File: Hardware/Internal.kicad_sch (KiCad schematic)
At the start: 128 parts, among them J1 SWD, J10 24V_OUT, J11 24V_OUT, J12 24V_OUT, J13 24V_OUT, J14 24V_OUT, J15 CAN, J16 CAN, J17 CAN, J18 CAN, J19 CAN, J2 CAN, J20 CAN, J21 DR16, J22 2.54, J23 2.54, J24 2.54, J3 USB_C_Receptacle_USB2.0, J4 JLINK_SWD, J5 CAN, J6 24V_IN, J7 24V_OUT, J8 24V_OUT, J9 24V_OUT, Q1 S8050, Q2 AO3400A, Q3 AO3400A, SW1 BTN1, SW2 RST, U1 STM32G431CBUx, U2 SIT1042T/3, U3 STM32F103CBT6, U4 RS3236, U5 RY8411, Y1 8MHz, Y3 8MHz

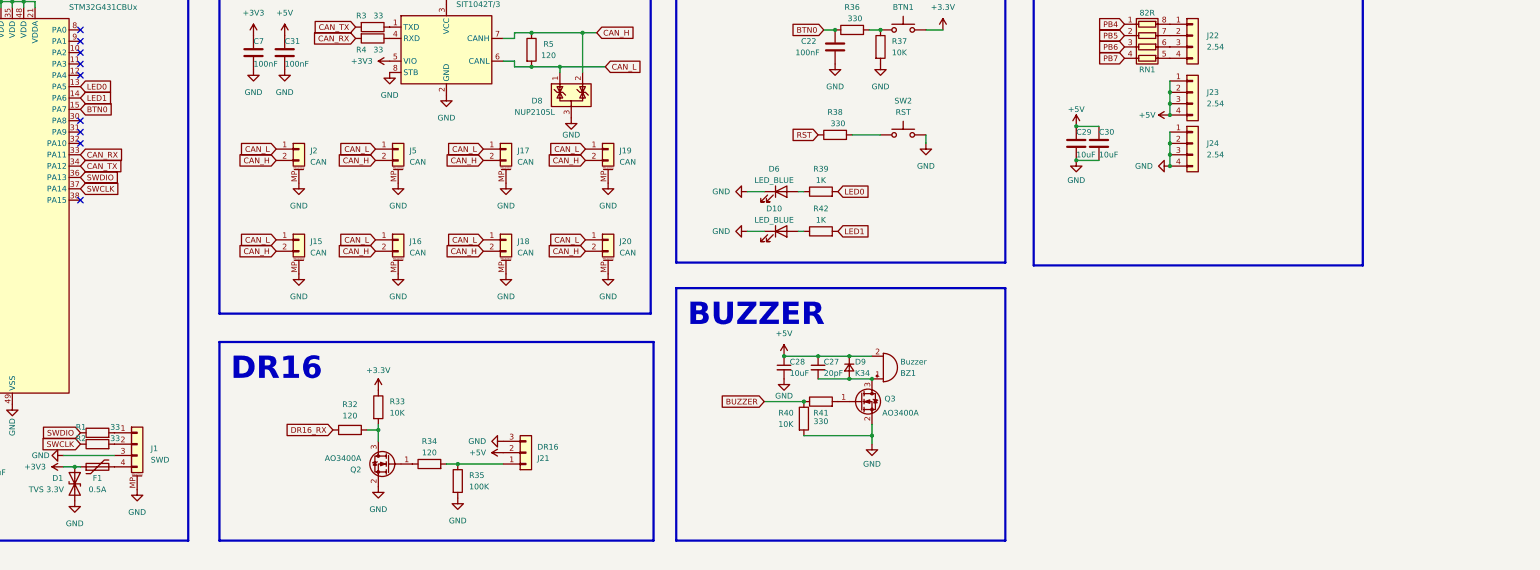
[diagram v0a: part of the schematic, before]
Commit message: update PCB
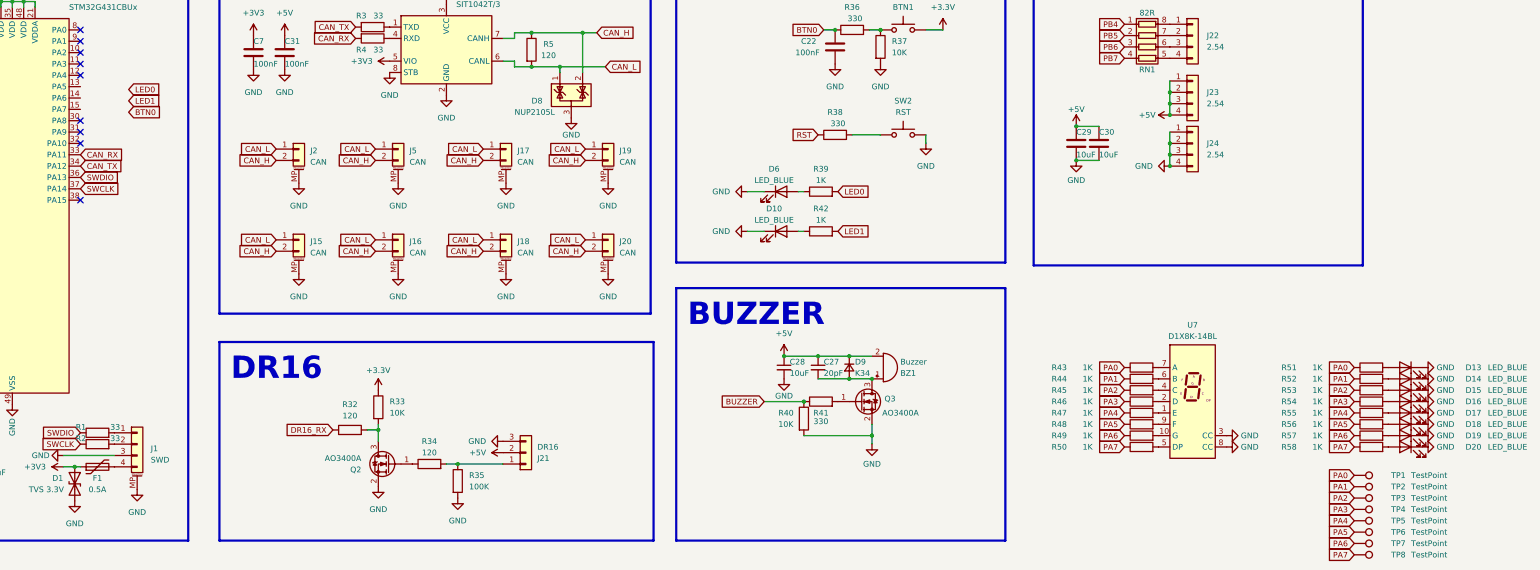
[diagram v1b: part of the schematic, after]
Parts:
- added D13, D14, D15, D16, D17, D18, D19, D20: LED_BLUE, LED_SMD:LED_0603_1608Metric, symbol Device:LED
- added R43, R44, R45, R46, R47, R48, R49, R50, R51, R52, R53, R54, R55, R56, R57, R58: 1K, Resistor_SMD:R_0603_1608Metric, symbol Device:R
- added TP1, TP2, TP3, TP4, TP5, TP6, TP7, TP8: TestPoint, TestPoint:TestPoint_THTPad_2.0x2.0mm_Drill1.0mm, symbol Connector:TestPoint
- added U7: D1X8K-14BL, Display_7Segment:D1X8K, symbol Display_Character:D1X8K-14BL
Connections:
- net BTN0: no longer U1.15 (PA7)
- net GND: now also D13.1 (K), D14.1 (K), D15.1 (K), D16.1 (K), D17.1 (K), D18.1 (K), D19.1 (K), D20.1 (K), U7.3 (CC), U7.8 (CC)
- net LED0: no longer U1.13 (PA5)
- net LED1: no longer U1.14 (PA6)
- new net: D20.2 (A), R58.2
- new net: R48.2, U7.9 (F)
- new net: D19.2 (A), R57.2
- new net: R46.2, U7.2 (D)
- new net: R49.2, U7.10 (G)
- new net: D15.2 (A), R53.2
- new net: R50.2, U7.5 (DP)
- new net: D17.2 (A), R55.2
- new net: D14.2 (A), R52.2
- new net: D13.2 (A), R51.2
- new net: R43.2, U7.7 (A)
- new net: D16.2 (A), R54.2
- new net: R47.2, U7.1 (E)
- new net: R45.2, U7.4 (C)
- new net: R44.2, U7.6 (B)
- new net: D18.2 (A), R56.2
- new net PA0: R43.1, R51.1, TP1.1
- new net PA1: R44.1, R52.1, TP2.1
- new net PA2: R45.1, R53.1, TP3.1
- new net PA3: R46.1, R54.1, TP4.1
- new net PA4: R47.1, R55.1, TP5.1
- new net PA5: R48.1, R56.1, TP6.1
- new net PA6: R49.1, R57.1, TP7.1
- new net PA7: R50.1, R58.1, TP8.1
